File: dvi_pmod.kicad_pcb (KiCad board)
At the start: 2 copper layers, 25 x 18.5 mm, 12 parts, among them J1 02x06, J2 Conn_01x02, J3 HDMI_A

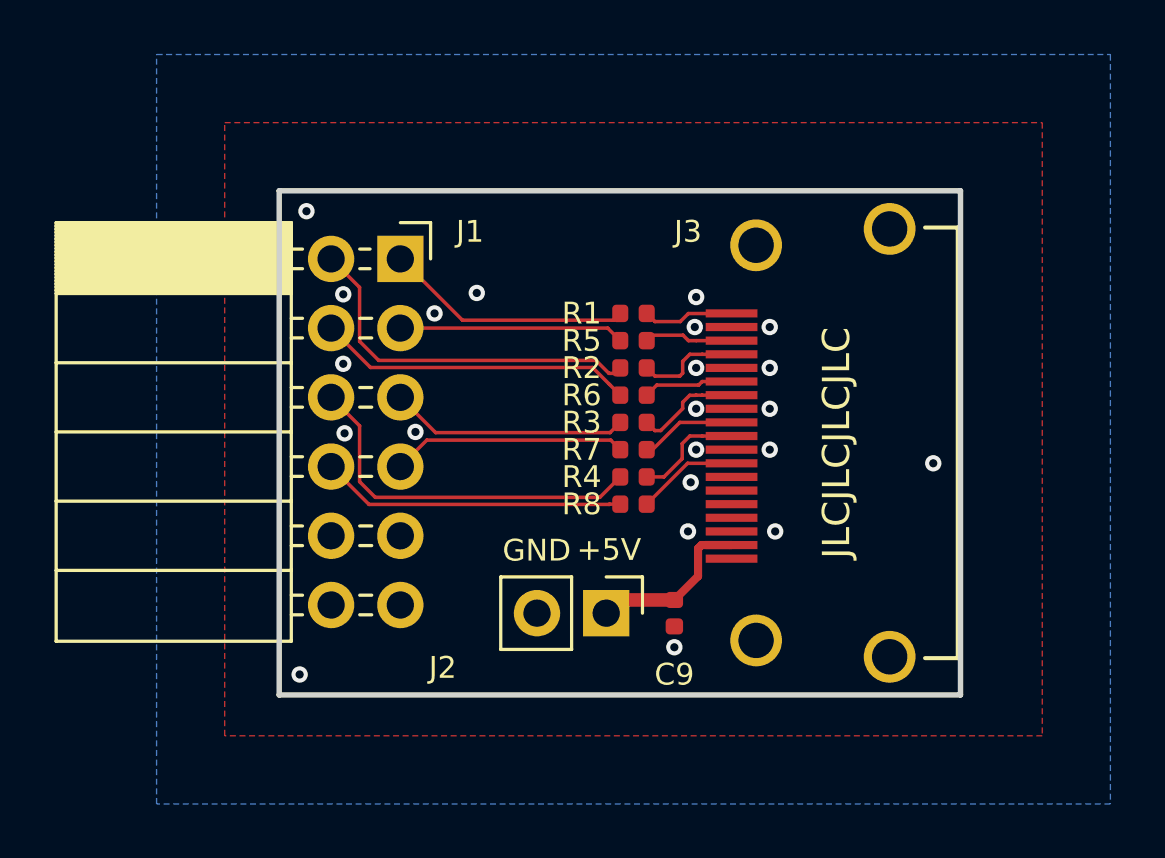
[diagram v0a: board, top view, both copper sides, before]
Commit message: Rev B board
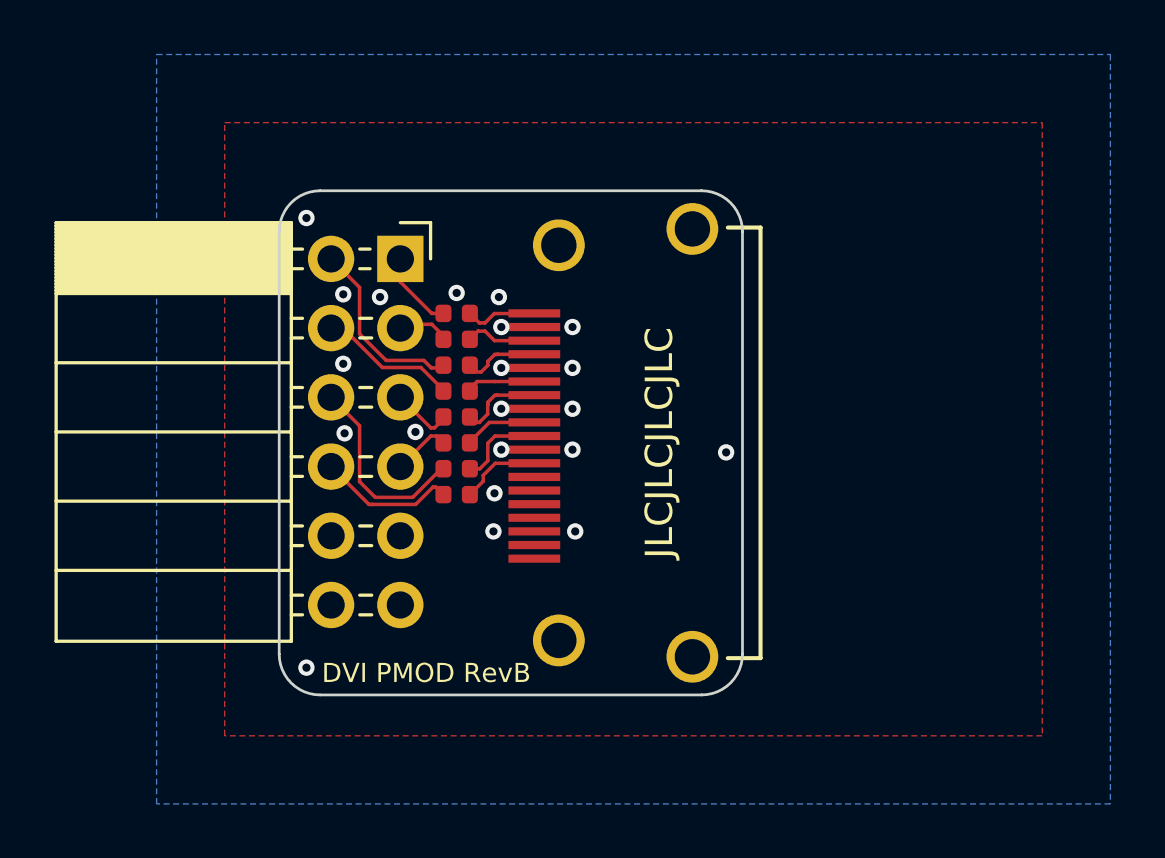
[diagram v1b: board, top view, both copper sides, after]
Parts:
- removed C9: 220n, Capacitor_SMD:C_0402_1005Metric
- removed J2: Conn_01x02, Connector_PinHeader_2.54mm:PinHeader_1x02_P2.54mm_Vertical
- J3: value HDMI_A -> NOT_HDMI_A
- moved J3 7.24 mm to (137.3, 76.8)
- moved R8 6.50 mm to (133.5, 78.7)
- moved R4 6.49 mm to (133.5, 77.7)
- moved R7 6.49 mm to (133.5, 76.8)
- moved R3 6.49 mm to (133.5, 75.8)
- moved R6 6.49 mm to (133.5, 74.8)
- moved R2 6.49 mm to (133.5, 73.9)
- moved R5 6.49 mm to (133.5, 73.0)
- moved R1 6.49 mm to (133.5, 72.0)
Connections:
- net Net-(J1-Pad11) renamed no_connect_18
- net Net-(J1-Pad12) renamed no_connect_19
- net Net-(J3-Pad13) renamed no_connect_20
- net Net-(J3-Pad14) renamed no_connect_21
- net Net-(J3-Pad15) renamed no_connect_22
- net Net-(J3-Pad16) renamed no_connect_23
- net Net-(J3-Pad19) renamed no_connect_25
- J3 pad 18: +5V -> no_connect_24
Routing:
- net /PMOD_D1+: track 13.6 -> 6.82 mm
- net /PMOD_D1-: track 11.6 -> 5.10 mm
- net /PMOD_D0+: track 8.76 -> 2.25 mm
- net /PMOD_D0-: track 8.62 -> 2.15 mm
- net /PMOD_CK+: track 13.6 -> 7.28 mm
- net /PMOD_D2-: track 8.26 -> 1.94 mm
- net +5V: track 6.23 -> 0.00 mm
- net /PMOD_D2+: track 9.11 -> 2.91 mm
- net /PMOD_CK-: track 11.2 -> 5.07 mm
- net /D1+: track 3.82 -> 2.78 mm
- net /D0-: track 3.53 -> 2.70 mm
- net /CK+: track 4.06 -> 3.24 mm
- net /D0+: track 3.91 -> 3.11 mm
- net /CK-: track 3.74 -> 2.97 mm
- net /D2+: track 3.36 -> 2.65 mm
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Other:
- board size 25 x 18.5 mm -> 17 x 18.5 mm
- net class Default removed
- board text added: "1"
- board text added: "12"
- board text added: "6"
- board text added: "7"
- board text added: "CK+"
- board text added: "CK-"
- board text added: "D0+"
- board text added: "D0-"
- board text added: "D1+"
- board text added: "D1-"
- board text added: "D2+"
- board text added: "D2-"
- board text added: "DVI PMOD RevB"
- board text added: "x"
- board text removed: "+5V"
